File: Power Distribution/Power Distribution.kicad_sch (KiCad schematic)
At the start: 14 parts, among them P1 ChargingBoardTP4056, SW1 Switch, U1 Raspberry Pi Zero 2 W, U2 Charging Board XL6009, U3 DAC MCP4922, U4 Audio Ampifier PAM8403D, U5 IMU BNO55

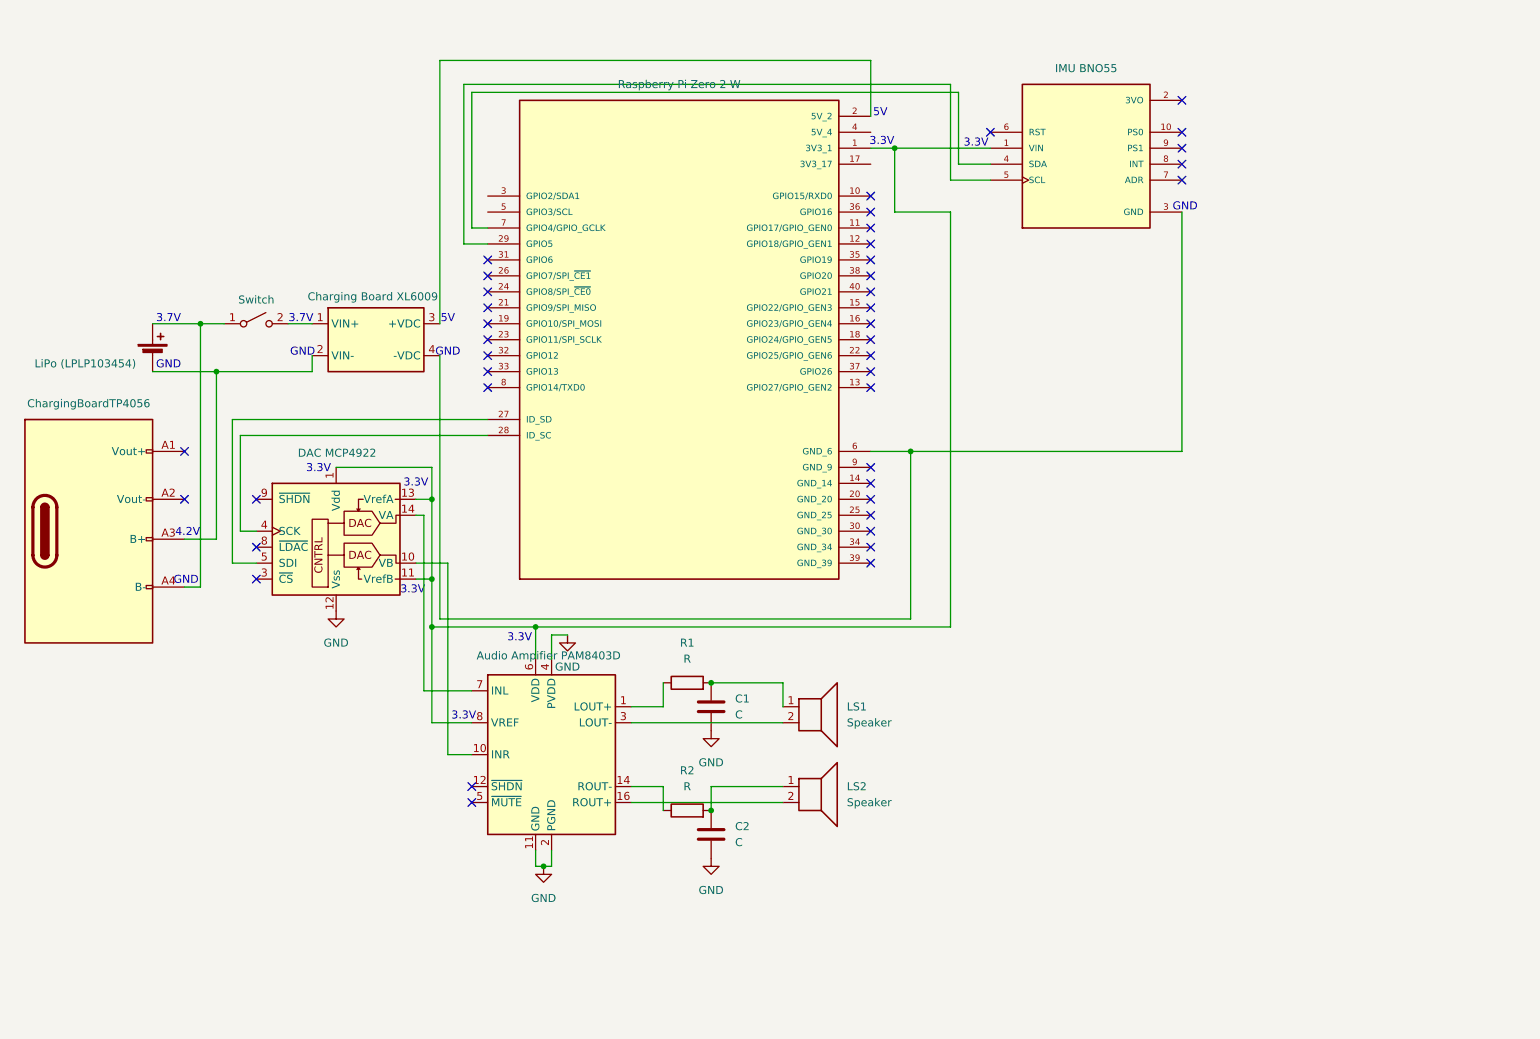
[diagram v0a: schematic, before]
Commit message: Updated the PCB schematic
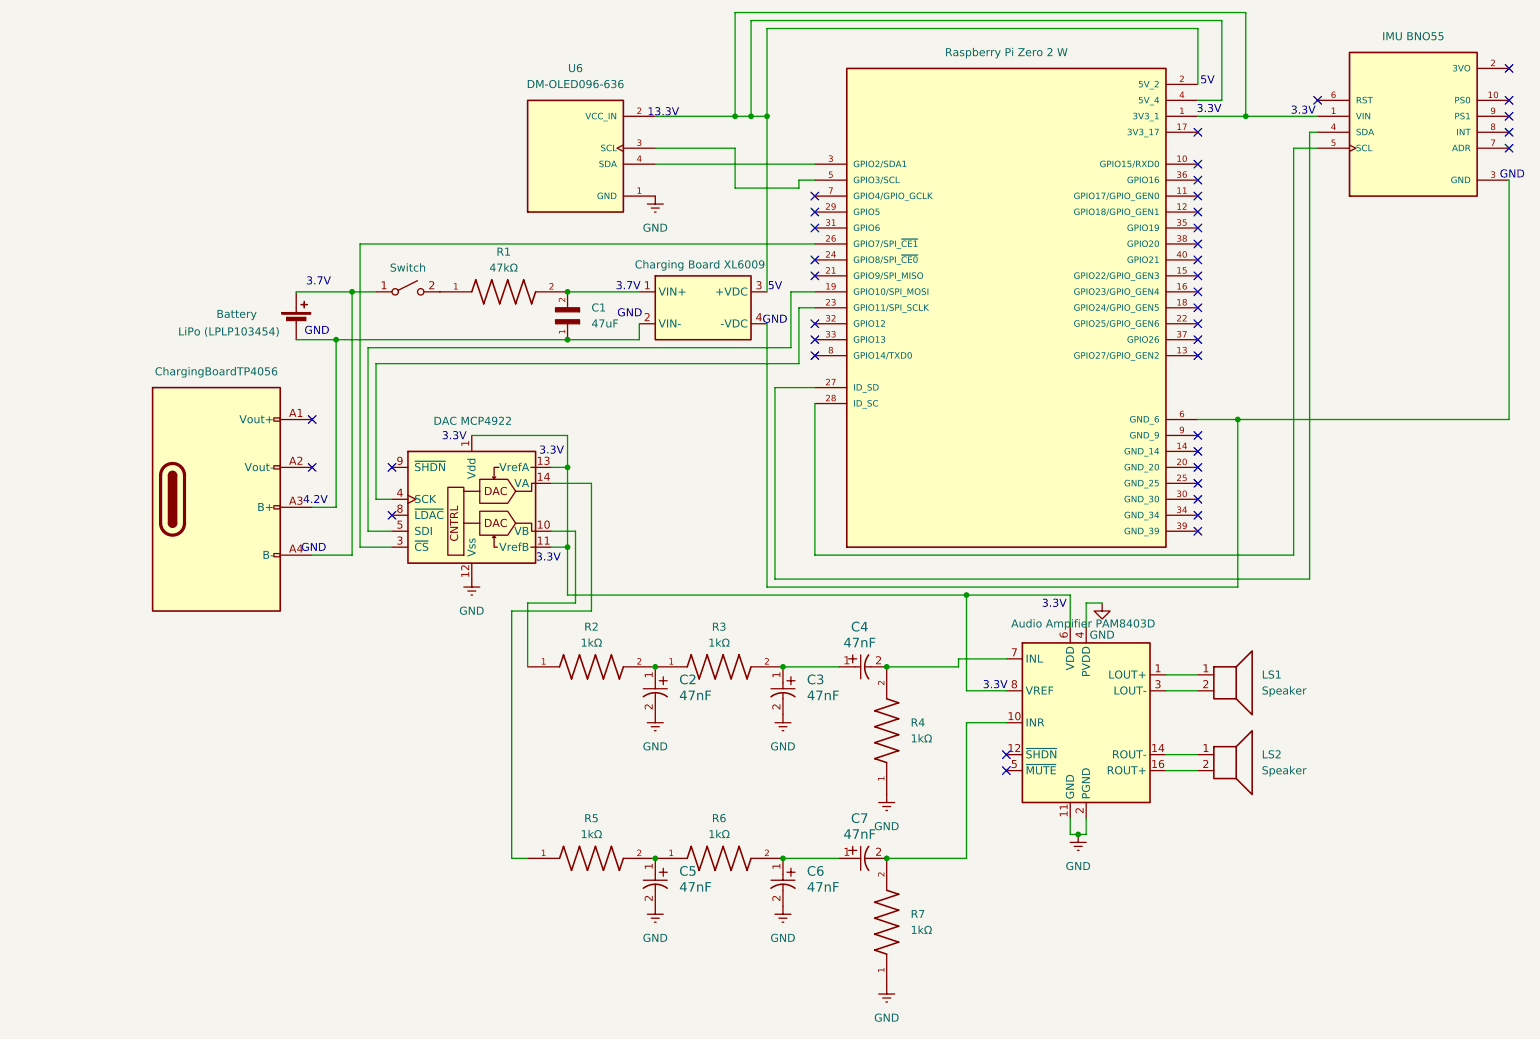
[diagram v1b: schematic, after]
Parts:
- removed C1, C2: C, symbol Device:C
- removed R1, R2: R, symbol Device:R
- added C1: 47uF, 47uF:CAPC3225X280N, symbol GCJ32ER70J476KE01L:GCJ32ER70J476KE01L
- added C2, C3, C4, C5, C6, C7: 47nF, 47nf:CAP_PAN_EEE_K16_PAN-L, symbol 2025-03-19_20-04-15:EEV-TG1A472M
- added R1: 47kΩ, 47k:RES_ERA6ARW473V, symbol ERA6ARW473V:ERA6ARW473V
- added R2, R3, R4, R5, R6, R7: 1kΩ, 1k:RES_ERJ2RKF1001X, symbol ERJ2RKF1001X:ERJ2RKF1001X
- added U6: DM-OLED096-636, OLED:MODULE_DM-OLED096-636, symbol DM-OLED096-636:DM-OLED096-636
- renumbered BT1 to Battery
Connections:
- net GND: now also C2.2, C3.2, C5.2, C6.2, R4.1, R7.1, U6.1 (GND)
- net at Battery.2 (-), P1.A3 (B+), U2.2 (+VDC)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: now also C1.1
- net at U2.1 (VIN+), U2.6 (VIN+): now also C1.2, R1.2; no longer SW1.2 (B)
- net at U3.1 (Vdd), U3.11 (VrefB), U3.13 (VrefA)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: no longer U1.1 (3V3_1), U5.1 (VIN)
- net at U1.19 (GPIO10/SPI_MOSI): now also U3.5 (SDI)
- net at U1.2 (5V_2), U2.2 (+VDC), U2.3 (+VDC): now also U1.1 (3V3_1), U1.4 (5V_4), U5.1 (VIN), U6.2 (VCC_IN)
- net at U1.23 (GPIO11/SPI_SCLK): now also U3.4 (SCK)
- net at U1.26 (GPIO7/SPI_~{CE1}): now also U3.3 (~{CS})
- net at U1.27 (ID_SD): now also U5.4 (SDA); no longer U3.5 (SDI)
- net at U1.28 (ID_SC): now also U5.5 (SCL); no longer U3.4 (SCK)
- net at U1.29 (GPIO5): no longer U5.5 (SCL)
- net at U1.3 (GPIO2/SDA1): now also U6.4 (SDA)
- net at U1.5 (GPIO3/SCL): now also U6.3 (SCL)
- net at U1.7 (GPIO4/GPIO_GCLK): no longer U5.4 (SDA)
- net at U4.1 (LOUT+): now also LS1.1
- net at U4.10 (INR): now also C7.2, R7.2; no longer U3.10 (VB)
- net at U4.14 (ROUT-): now also LS2.1
- net at U4.7 (INL): now also C4.2, R4.2; no longer U3.14 (VA)
- new net: C5.1, R5.2, R6.1
- new net: C6.1, C7.1, R6.2
- new net: R1.1, SW1.2 (B)
- new net: C3.1, C4.1, R3.2
- new net: R2.1, U3.10 (VB)
- new net: R5.1, U3.14 (VA)
- new net: C2.1, R2.2, R3.1
- no-connect marks 42 -> 41
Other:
- note added: "13.3V"
- company: (none) -> VISION
- title: (none) -> Proposed Power Distribution Schematics
- moved on the sheet: LS1, LS2
